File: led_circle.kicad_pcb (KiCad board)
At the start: 2 copper layers, 50 x 50 mm, 22 parts, among them P1 CONN_01X11, U1 TLC5940

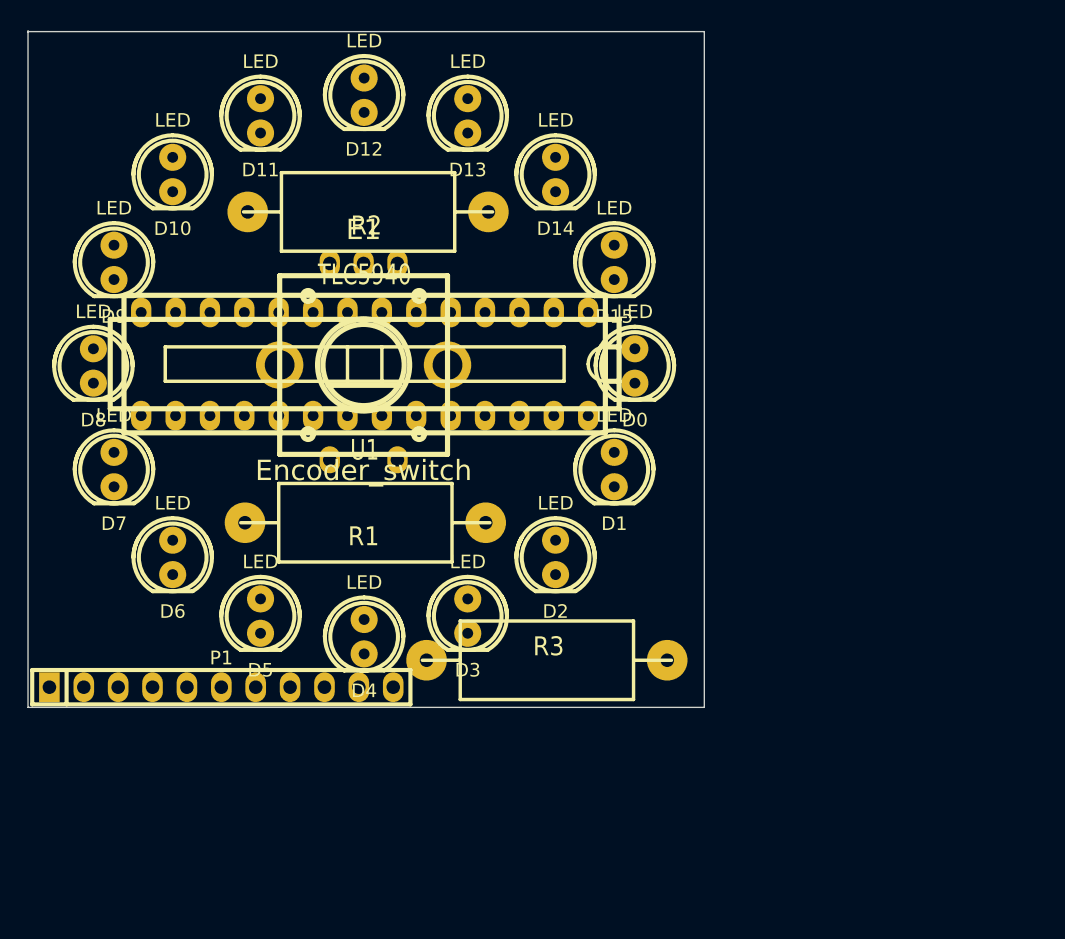
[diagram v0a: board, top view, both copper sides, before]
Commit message: some various changes and missing stuff
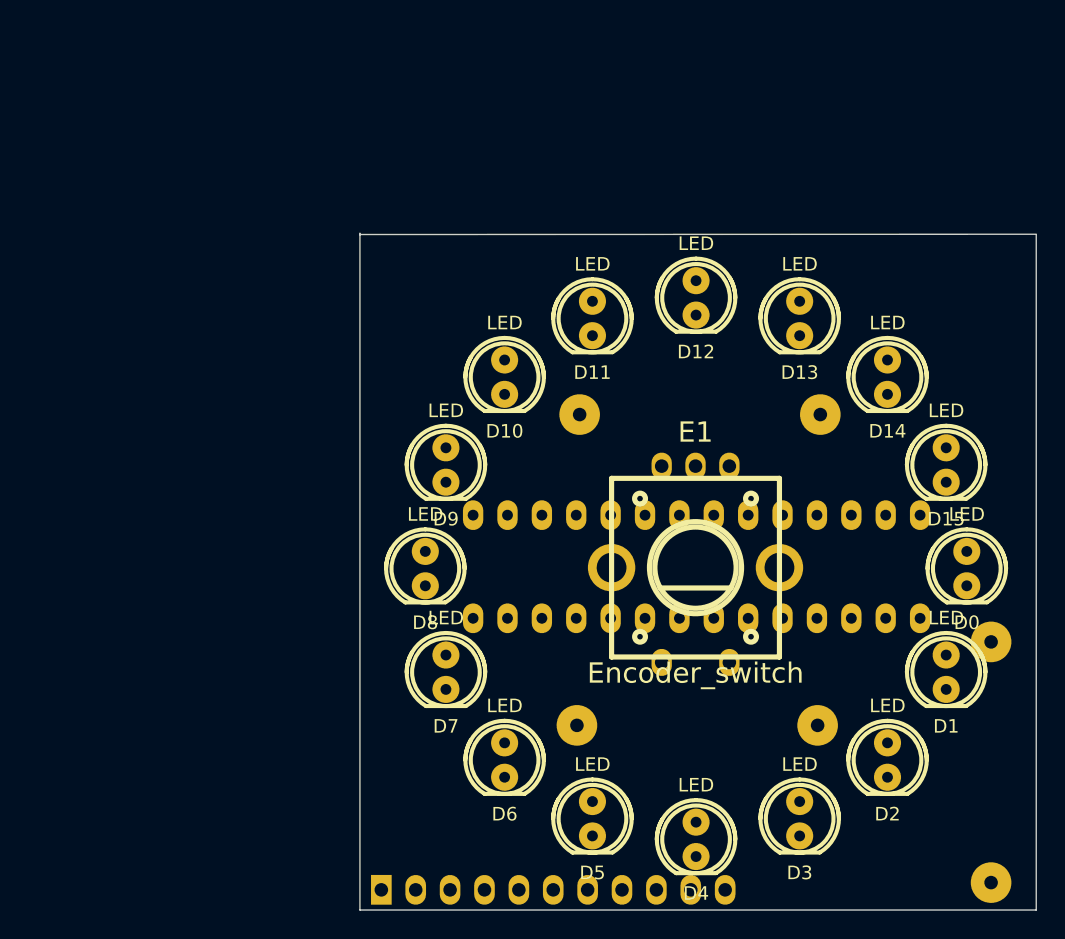
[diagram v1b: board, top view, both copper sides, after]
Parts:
- P1, R1, R2, R3, U1: moved to B.Cu
- moved R3 33.7 mm to (83.2, 66.1), turned to 270 degrees
- moved D0 28.7 mm to (81.4, 51.8)
- moved D12 28.7 mm to (61.4, 31.8)
- moved D6 28.7 mm to (47.3, 66.0)
- moved D7 28.7 mm to (42.9, 59.5)
- moved D8 28.7 mm to (41.4, 51.8)
- moved E1 28.7 mm to (61.4, 51.8)
- moved R2 28.7 mm to (61.7, 40.4)
- moved U1 28.7 mm to (61.5, 51.7)
- moved D1 28.7 mm to (79.9, 59.5)
- moved D11 28.7 mm to (53.8, 33.3)
- moved D13 28.7 mm to (69.1, 33.3)
- moved D2 28.7 mm to (75.6, 66.0)
- moved D5 28.7 mm to (53.8, 70.3)
- moved D14 28.7 mm to (75.6, 37.7)
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
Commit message: forgot to commit all the changes...
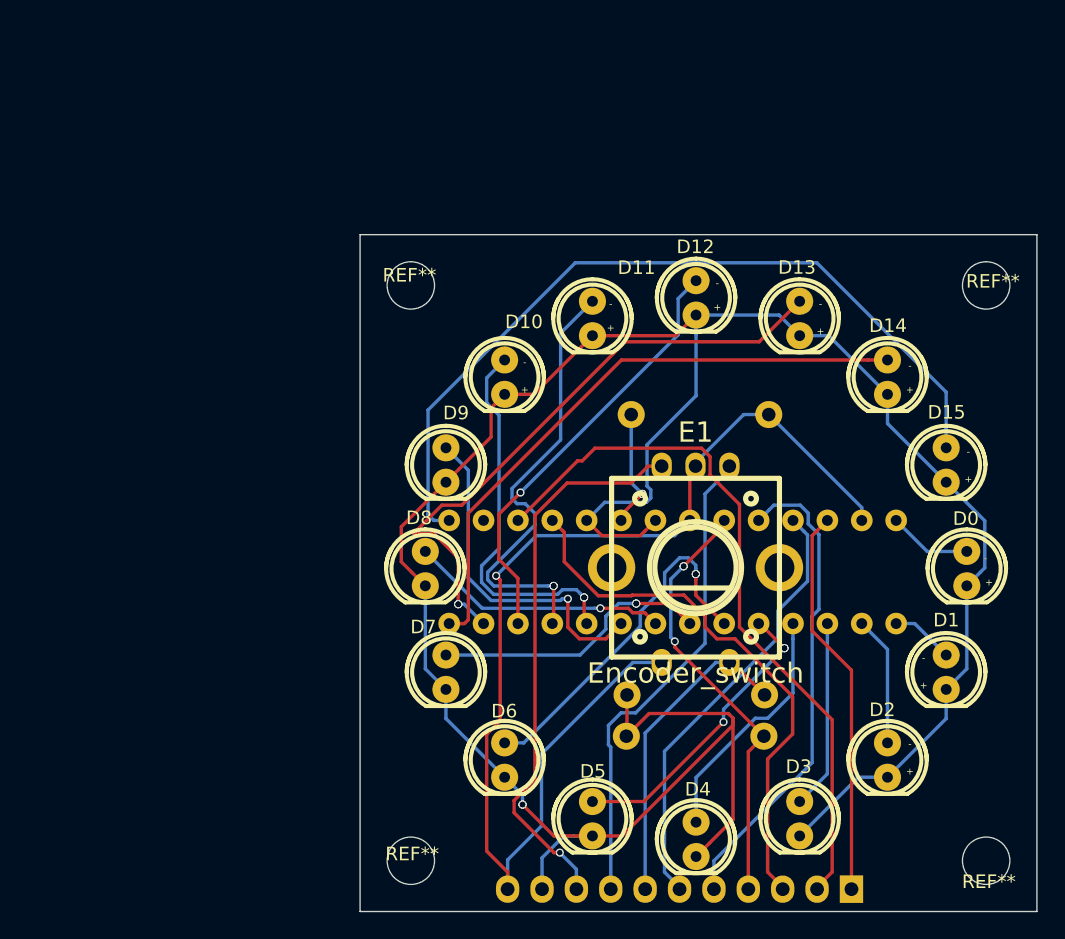
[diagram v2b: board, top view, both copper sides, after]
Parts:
- added REF**: MountingHole_3-5mm, Mounting_Holes:MountingHole_3-5mm, F.Cu at (82.8, 30.9)
- added REF**: MountingHole_3-5mm, Mounting_Holes:MountingHole_3-5mm, F.Cu at (40.4, 30.9)
- added REF**: MountingHole_3-5mm, Mounting_Holes:MountingHole_3-5mm, F.Cu at (82.8, 73.4)
- added REF**: MountingHole_3-5mm, Mounting_Holes:MountingHole_3-5mm, F.Cu at (40.4, 73.4)
- P1: value CONN_01X11 -> CONN_11; footprint w_pin_strip:pin_strip_11 -> Pin_Headers:Pin_Header_Straight_1x11
- R1, R2, R3: footprint w_pth_resistors:R12x5.2 -> Resistors_ThroughHole:Resistor_Horizontal_RM10mm
- U1: footprint w_pth_circuits:dil_28-300_socket -> Housings_DIP:DIP-28_W7.62mm
- moved R3 22.4 mm to (61.4, 61.1), turned to 0 degrees
- moved P1 22.0 mm to (72.9, 75.5), turned to 90 degrees
- moved U1 15.3 mm to (76.2, 55.9), turned to 90 degrees
- moved R1 0.82 mm to (61.4, 64.2)
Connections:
- E1 pad 2: GNDREF -> GND
- E1 pad 4: GNDREF -> GND
- P1 pad 10: /VCC -> +5V
- P1 pad 11: /GND -> GND
- R2 pad 1: GNDREF -> GND
- U1 pad 22: GNDREF -> GND
- U1 pad 27: GNDREF -> GND
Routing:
- net +5V: track 0.00 -> 189.7 mm, vias 0 -> 2
- net GND: track 0.00 -> 85.0 mm, vias 0 -> 1
- net Net-(D15-Pad1): track 0.00 -> 60.3 mm
- net /SOUT: track 0.00 -> 52.8 mm
- net Net-(D13-Pad1): track 0.00 -> 45.6 mm, vias 0 -> 2
- net Net-(D14-Pad1): track 0.00 -> 45.1 mm
- net /ENC_B: track 0.00 -> 41.3 mm, vias 0 -> 1
- net /GSCLK: track 0.00 -> 40.4 mm
- net /XLAT: track 0.00 -> 35.7 mm
- net /ENC_A: track 0.00 -> 35.7 mm
- net Net-(D11-Pad1): track 0.00 -> 33.4 mm, vias 0 -> 2
- net /SCLK: track 0.00 -> 32.5 mm
- net /BLANK: track 0.00 -> 32.2 mm, vias 0 -> 3
- net Net-(D12-Pad1): track 0.00 -> 31.9 mm, vias 0 -> 1
- net /SIN: track 0.00 -> 28.9 mm
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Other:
- outline, holes or cut-outs redrawn
- board text added: "+"
- board text added: "+5"
- board text added: "-"
- board text added: "1"
- board text added: "10"
- board text added: "10k"
- board text added: "11"
- board text added: "12"
- board text added: "13"
- board text added: "14"
- board text added: "15"
- board text added: "16"
- board text added: "17"
- board text added: "18"
- board text added: "19"
- board text added: "2"
- board text added: "2.2k"
- board text added: "20"
- board text added: "21"
- board text added: "22"
- board text added: "23"
- board text added: "24"
- board text added: "25"
- board text added: "26"
- board text added: "27"
- board text added: "28"
- board text added: "3"
- board text added: "4"
- board text added: "5"
- board text added: "6"
- board text added: "7"
- board text added: "8"
- board text added: "9"
- board text added: "BLANK"
- board text added: "ENC_A"
- board text added: "ENC_B"
- board text added: "ENC_PB"
- board text added: "Encoder led board"
- board text added: "GND"
- board text added: "GSCLK"
- board text added: "SCLK"
- board text added: "SIN"
- board text added: "SOUT"
- board text added: "TLC5940"
- board text added: "XLAT"
- board text added: "gnd"
- board text added: "jjrh (2015)"
- board text added: "rev.1"
